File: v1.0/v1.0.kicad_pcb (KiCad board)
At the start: 2 copper layers, 130.3 x 84.8 mm, 46 parts, among them J1 MJ-4PP-9, SW1 SW_PUSH, SW10 SW_PUSH, SW11 SW_PUSH, SW12 SW_PUSH, SW13 SW_PUSH, SW14 SW_PUSH, SW15 SW_PUSH, SW16 SW_PUSH, SW17 SW_PUSH, SW18 SW_PUSH, SW19 SW_PUSH, SW2 SW_PUSH, SW20 SW_PUSH, SW3 SW_PUSH, SW4 SW_PUSH, SW5 SW_PUSH, SW6 SW_PUSH, SW7 SW_PUSH, SW8 SW_PUSH, SW9 SW_PUSH, U1 ProMicro

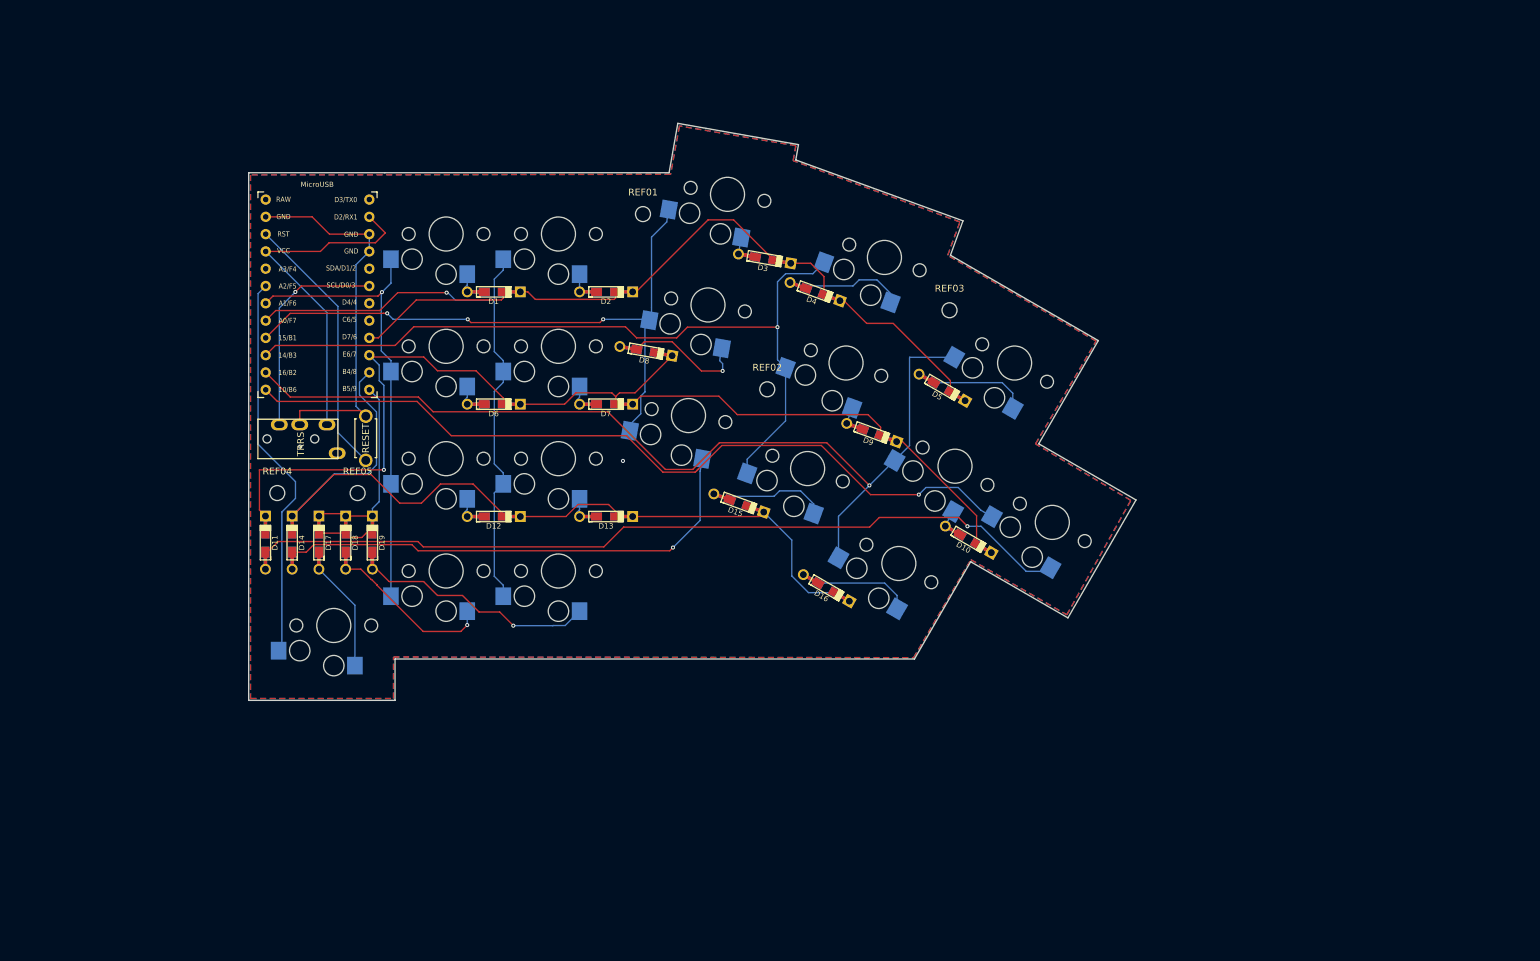
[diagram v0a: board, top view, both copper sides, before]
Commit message: updated
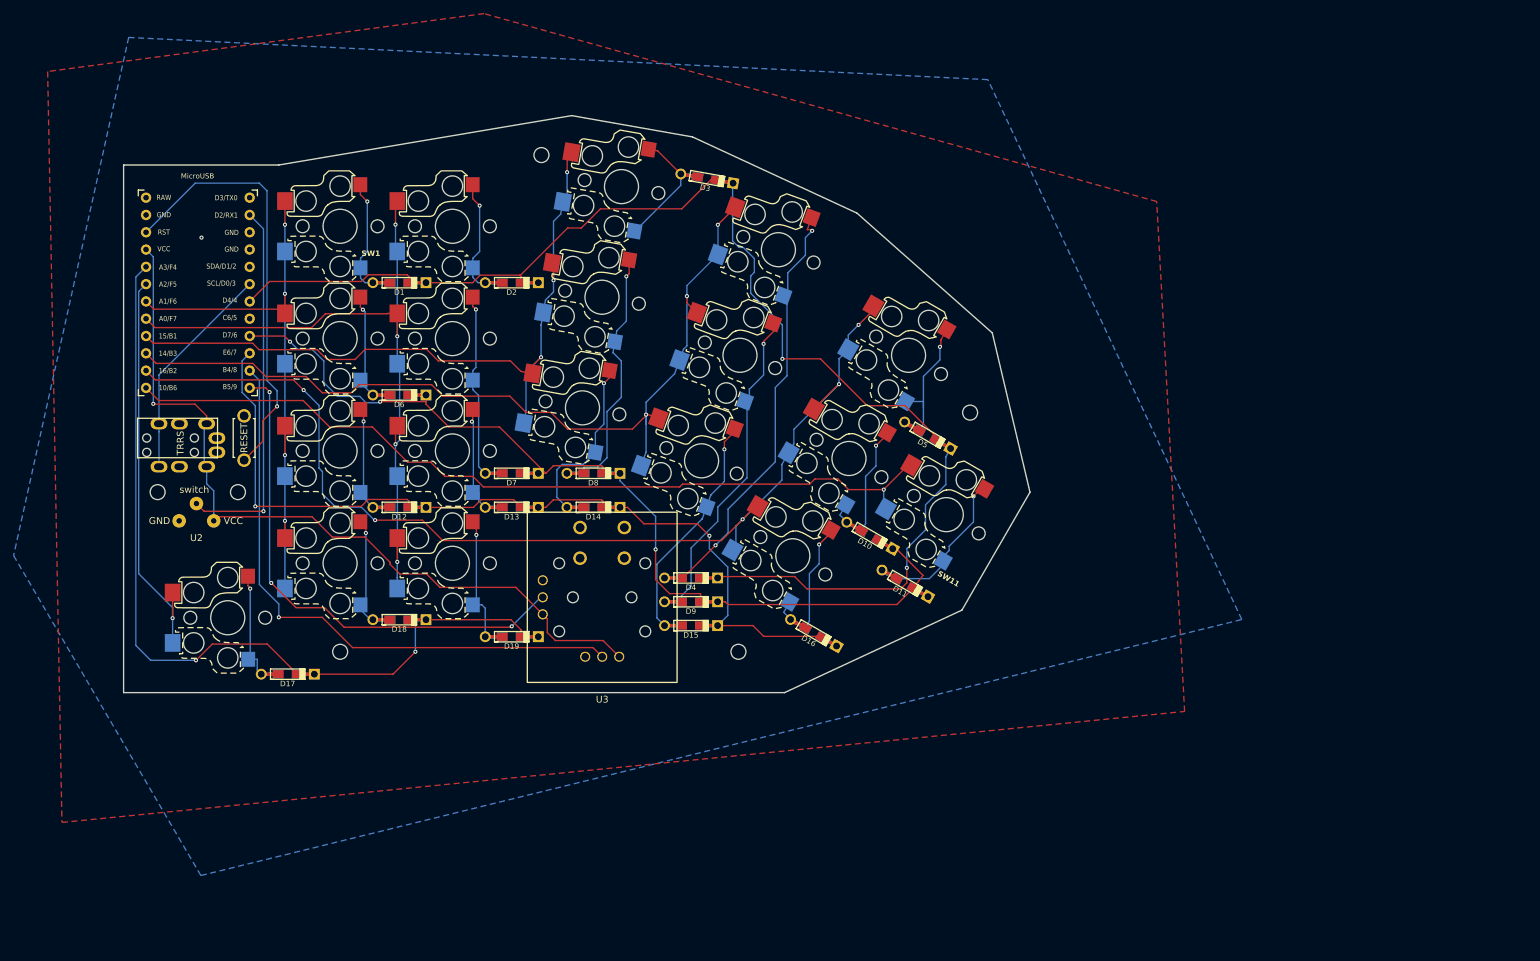
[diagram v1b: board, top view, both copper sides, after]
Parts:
- added REF06: MountingHole_2.2mm_M2, MountingHole:MountingHole_2.2mm_M2, F.Cu at (148.2, 129.9)
- added U2: switch, otborad:triangle, F.Cu at (68.6, 110.7)
- added U3: RKJXV122400R, otborad:RKJXV122400R, F.Cu at (128.2, 121.9)
- J1: footprint kbd:MJ-4PP-9 -> otborad:MJ-4PP-9_reversible
- SW1, SW10, SW11, SW12, SW13, SW14, SW15, SW16, SW17, SW18, SW19, SW2, SW3, SW4, SW5, SW6, SW7, SW8, SW9: footprint footprint:keyswitch_choc12_hotswap_1u_rev -> otborad:choc1_0.8u_reversible
- U1: footprint footprint:ProMicro -> otborad:ProMicro
- moved REF04 102.4 mm to (182.2, 94.8)
- moved D11 94.1 mm to (172.6, 119.9), turned to -30 degrees
- moved REF01 82.2 mm to (62.9, 106.5)
- moved REF02 79.2 mm to (74.7, 106.5)
- moved REF03 64.1 mm to (119.2, 57.0)
- moved D4 45.8 mm to (141.2, 119.1), turned to 0 degrees
- moved D14 44.6 mm to (126.9, 108.7), turned to 0 degrees
- moved D9 36.4 mm to (141.2, 122.6), turned to 0 degrees
- moved D19 24.7 mm to (114.9, 127.7), turned to 0 degrees
- moved REF05 23.5 mm to (89.7, 129.9)
- moved D17 19.9 mm to (82.0, 133.2), turned to 0 degrees
- moved D8 19.5 mm to (126.9, 103.7), turned to 0 degrees
- moved D15 19.3 mm to (141.2, 126.1), turned to 0 degrees
- moved SW20 17.9 mm to (75.6, 98.5)
- moved J1 17.7 mm to (59.8, 98.5)
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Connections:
- U1 pad 10: row2 -> row3
- U1 pad 11: row3 -> VRx
- U1 pad 12: row4 -> VRy
- U1 pad 2: pwr -> switch
- U1 pad 20: unconnected-(U1-F4/A3-Pad20) -> row4
- U1 pad 7: unconnected-(U1-4/D4-Pad7) -> row1
- U1 pad 9: row1 -> row2
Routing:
- net Net-(D11-A): track 121.7 -> 27.0 mm
- net row1: track 119.9 -> 211.3 mm, vias 0 -> 2
- net VRx: track 0.00 -> 87.9 mm, vias 0 -> 1
- net row4: track 49.4 -> 135.2 mm, vias 0 -> 2
- net VRy: track 0.00 -> 75.7 mm, vias 0 -> 3
- net pwr: track 51.2 -> 117.5 mm, vias 0 -> 1
- net GND: track 56.5 -> 0.00 mm, vias 2 -> 1
- net switch: track 0.00 -> 54.7 mm, vias 0 -> 1
- net Net-(D4-A): track 17.5 -> 66.7 mm, vias 0 -> 2
- net Net-(D14-A): track 76.7 -> 30.7 mm
- net Net-(D9-A): track 8.89 -> 51.8 mm, vias 0 -> 1
- net reset: track 39.3 -> 63.4 mm, vias 0 -> 1
- net Net-(D7-A): track 8.10 -> 32.1 mm, vias 0 -> 1
- net Net-(D15-A): track 17.4 -> 38.8 mm, vias 0 -> 1
- net Net-(D19-A): track 44.1 -> 23.8 mm
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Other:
- board size 130.3 x 84.8 mm -> 133.1 x 84.8 mm

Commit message: updated
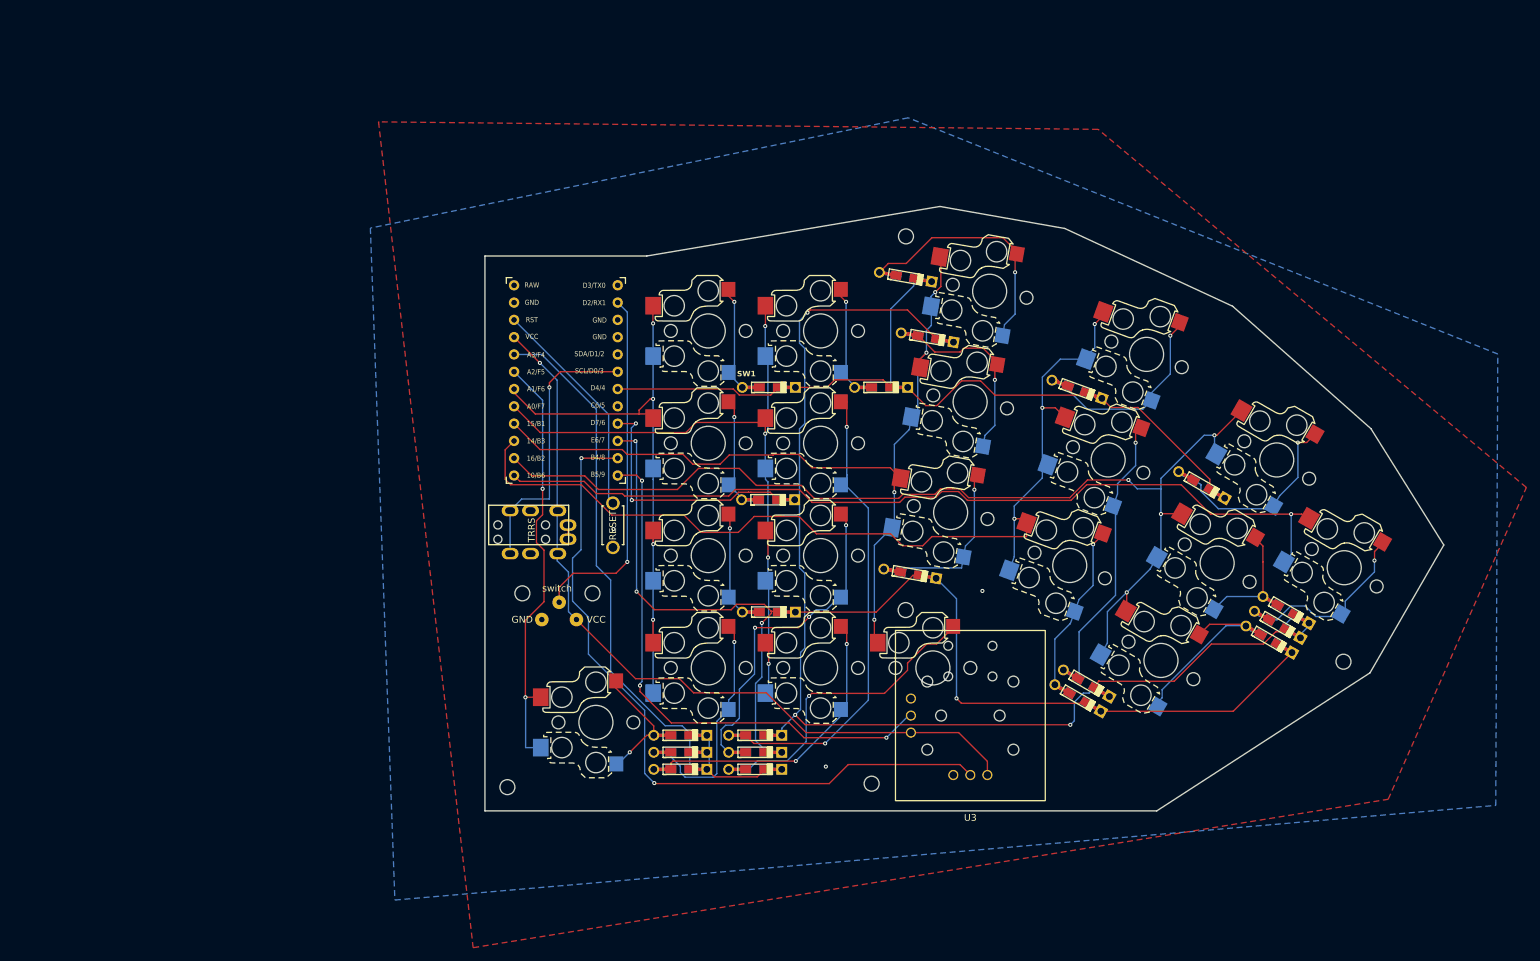
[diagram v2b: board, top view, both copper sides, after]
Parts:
- added D20: D, Keebio-Parts:Diode-dual, F.Cu at (150.6, 147.2)
- added REF07: MountingHole_2.2mm_M2, MountingHole:MountingHole_2.2mm_M2, F.Cu at (126.7, 121.4)
- added SW21: SW_PUSH, kbd:ResetSW, F.Cu at (129.7, 111.4)
- SW20: footprint kbd:ResetSW -> otborad:choc1_0.8u_reversible_uponly
- U3: value RKJXV122400R -> RKJXV122400R_1; footprint otborad:RKJXV122400R -> otborad:RKJXV122400R_1
- moved REF05 147.4 mm to (237.0, 131.4)
- moved REF01 111.2 mm to (172.7, 123.8)
- moved SW20 106.7 mm to (176.7, 132.3), turned to 0 degrees
- moved REF02 102.5 mm to (167.7, 149.3)
- moved REF04 87.4 mm to (114.2, 149.8)
- moved D16 66.9 mm to (226.1, 128.1)
- moved D4 63.1 mm to (197.9, 91.4), turned to -20 degrees
- moved D10 62.1 mm to (228.6, 123.8)
- moved D9 59.3 mm to (199.3, 134.6), turned to -30 degrees
- moved SW11 59.0 mm to (237.1, 117.6)
- moved D17 58.4 mm to (139.6, 142.2)
- moved D15 57.8 mm to (198.0, 136.7), turned to -30 degrees
- moved U3 56.8 mm to (182.2, 139.3)
- moved D1 56.4 mm to (152.6, 91.1)
- moved D12 56.4 mm to (152.6, 124.1)
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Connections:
- SW20 pad 1: reset -> col4
- SW20 pad 2: GND -> Net-(D20-A)
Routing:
- net row2: track 161.2 -> 238.5 mm, vias 3 -> 5
- net row1: track 211.3 -> 135.1 mm, vias 2 -> 0
- net Net-(D20-A): track 0.00 -> 48.6 mm, vias 0 -> 1
- net Net-(D7-A): track 32.1 -> 74.0 mm, vias 1 -> 2
- net row3: track 144.6 -> 185.4 mm, vias 2 -> 4
- net Net-(D4-A): track 66.7 -> 33.1 mm, vias 2 -> 1
- net Net-(D13-A): track 21.1 -> 54.0 mm, vias 1 -> 3
- net reset: track 63.4 -> 32.9 mm, vias 1 -> 0
- net row4: track 135.2 -> 108.7 mm, vias 2 -> 0
- net Net-(D19-A): track 23.8 -> 47.6 mm, vias 1 -> 2
- net VRx: track 87.9 -> 106.8 mm, vias 1 -> 2
- net col4: track 108.4 -> 127.2 mm, vias 3 -> 4
- net Net-(D3-A): track 22.7 -> 40.4 mm, vias 0 -> 1
- net Net-(D18-A): track 21.8 -> 37.4 mm
- net col5: track 129.9 -> 143.5 mm
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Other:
- board size 133.1 x 84.8 mm -> 140.8 x 88.8 mm
